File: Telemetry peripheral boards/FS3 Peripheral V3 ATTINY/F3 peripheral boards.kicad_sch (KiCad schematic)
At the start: 49 parts, among them J1 ATS668LSM, J2 Exit Connector, J3 Potentiometer, J4 Strain Gauge, J5 Tire temp Sensor, J6 1x1 Tire Air Temp Sensor, J7 1x8 Tire Surface Temp Sensor, U1 LM2907M/NOPB, U2 INA125U, U3 MCP2515-I/SO, U4 ISO1050DUB, U5 ATtiny1616-S, U6 LM7805CV, U7 LF33CV, Y1 STDCSU1-8M

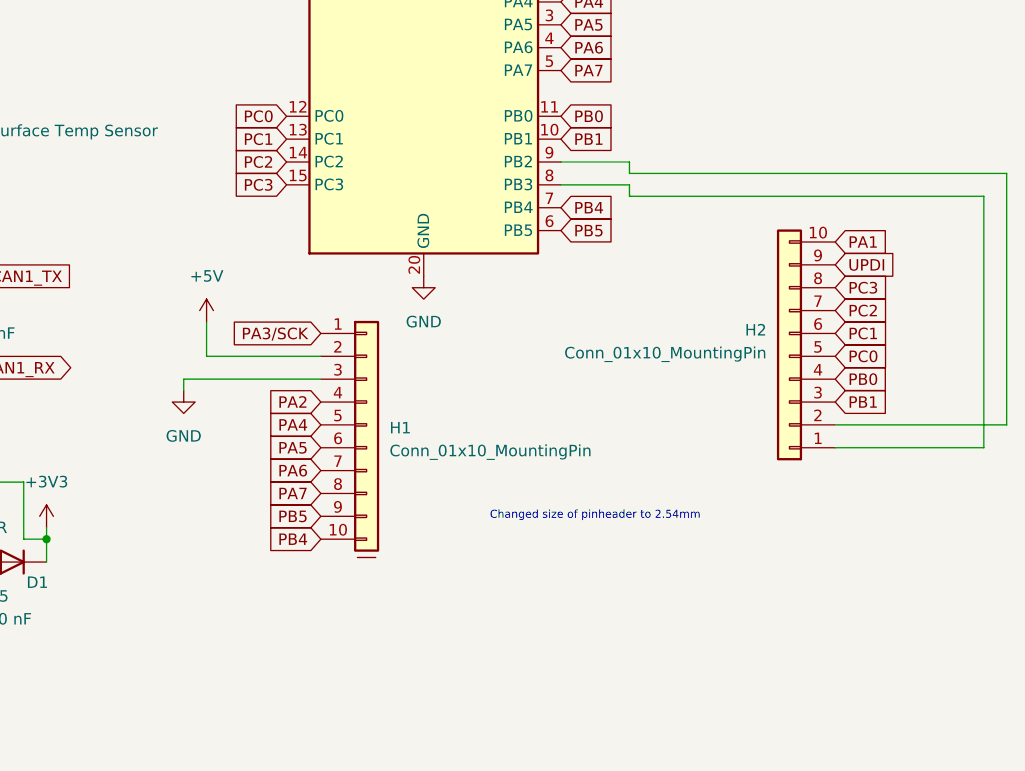
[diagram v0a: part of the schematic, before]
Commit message: updated schematic
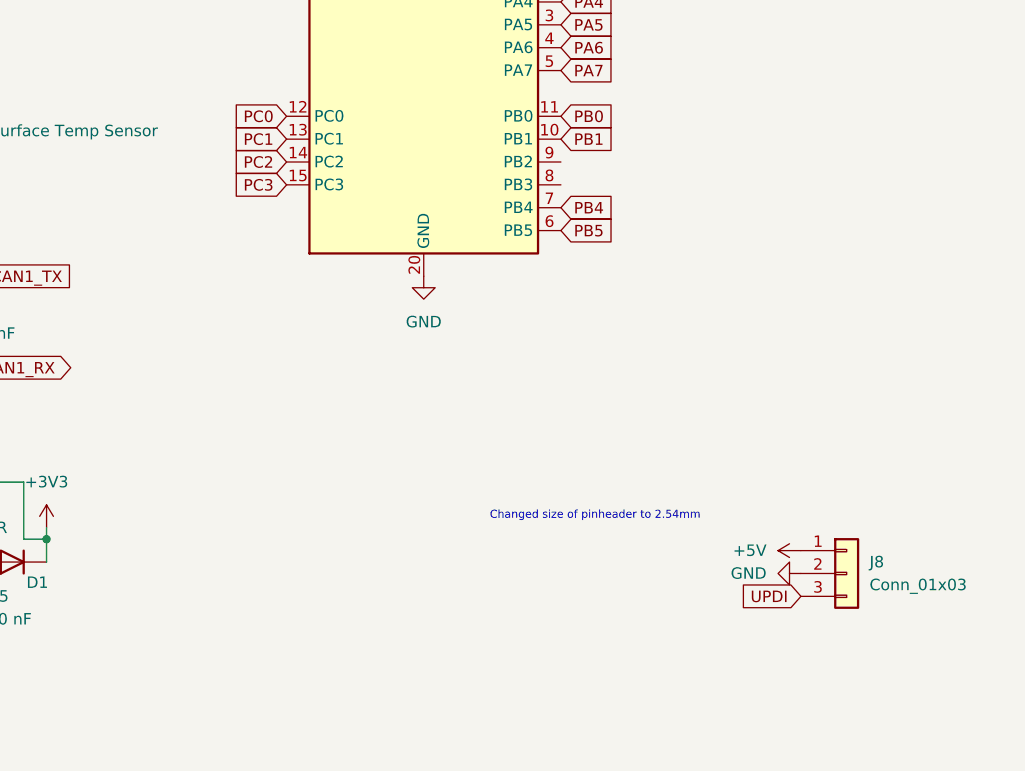
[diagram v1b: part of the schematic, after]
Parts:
- removed H1, H2: Conn_01x10_MountingPin, Connector_PinHeader_2.54mm:PinHeader_1x10_P2.54mm_Vertical, symbol Connector_Generic_MountingPin:Conn_01x10_MountingPin
- added J8: Conn_01x03, Connector_PinHeader_2.54mm:PinHeader_1x03_P2.54mm_Vertical, symbol Connector_Generic:Conn_01x03
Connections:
- net +5V: now also J8.1 (Pin_1)
- net GND: now also J8.2 (Pin_2)
- net UPDI: now also J8.3 (Pin_3)

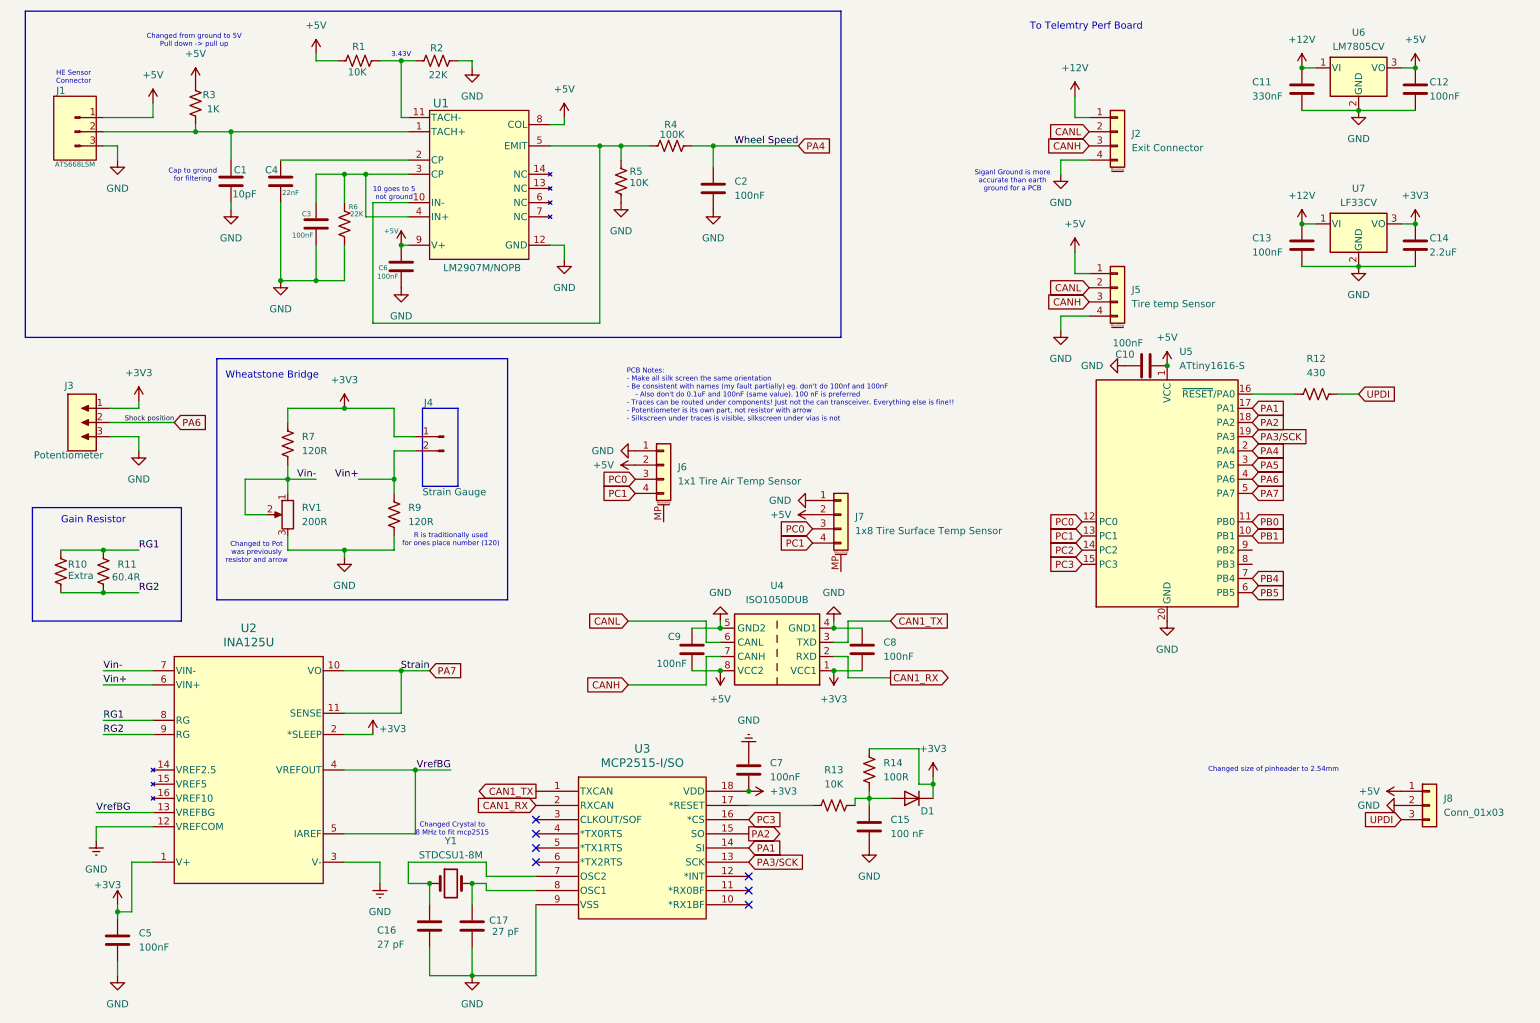
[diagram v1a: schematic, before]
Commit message: added testing pin headers and made pin change on attiny v3
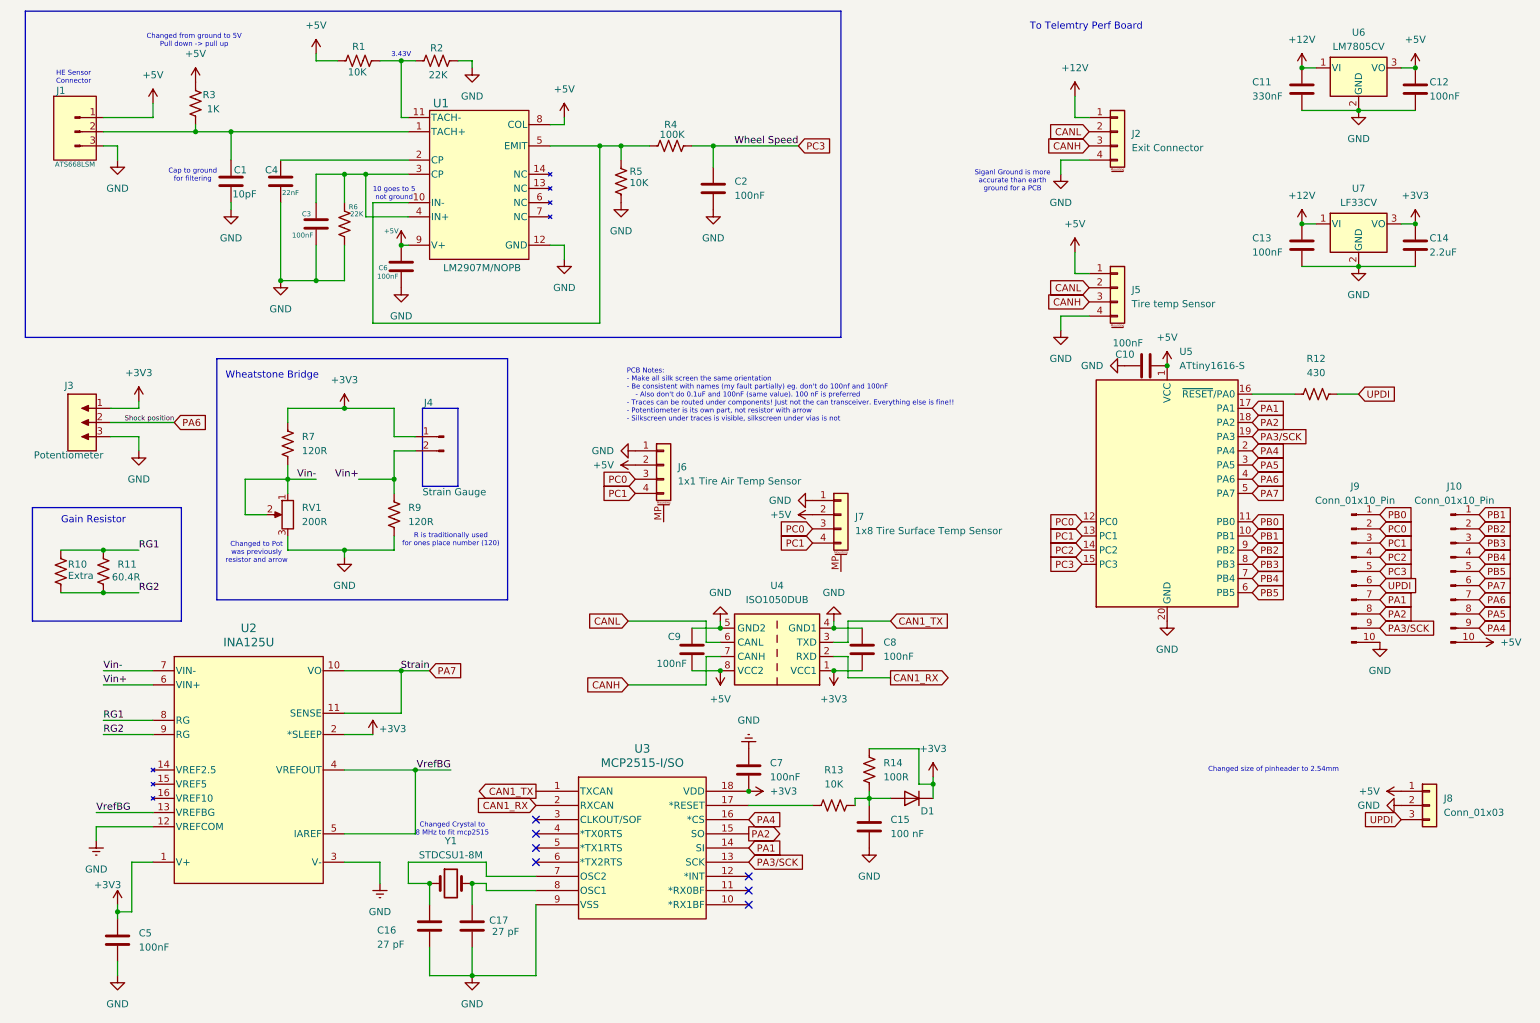
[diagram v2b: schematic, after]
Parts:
- added J10, J9: Conn_01x10_Pin, Connector_PinHeader_2.00mm:PinHeader_1x10_P2.00mm_Vertical, symbol Connector:Conn_01x10_Pin
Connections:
- net +5V: now also J10.10 (Pin_10)
- net GND: now also J9.10 (Pin_10)
- net PA1: now also J9.7 (Pin_7)
- net PA2: now also J9.8 (Pin_8)
- net PA3/SCK: now also J9.9 (Pin_9)
- net PA4: now also U3.16 (*CS), J10.9 (Pin_9); no longer C2.1, R4.2
- net PA5: now also J10.8 (Pin_8)
- net PA6: now also J10.7 (Pin_7)
- net PA7: now also J10.6 (Pin_6)
- net PB0: now also J9.1 (Pin_1)
- net PB1: now also J10.1 (Pin_1)
- net PB4: now also J10.4 (Pin_4)
- net PB5: now also J10.5 (Pin_5)
- net PC0: now also J9.2 (Pin_2)
- net PC1: now also J9.3 (Pin_3)
- net PC2: now also J9.4 (Pin_4)
- net PC3: now also C2.1, R4.2, J9.5 (Pin_5); no longer U3.16 (*CS)
- net UPDI: now also J9.6 (Pin_6)
- net PB3: now reaches U5.8 (PB3)
- net PB3: now also J10.3 (Pin_3)
- net PB2: now reaches U5.9 (PB2)
- net PB2: now also J10.2 (Pin_2)

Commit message: fixed attiny v3
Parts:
- J10, J9: footprint Connector_PinHeader_2.00mm:PinHeader_1x10_P2.00mm_Vertical -> Connector_PinHeader_2.54mm:PinHeader_1x10_P2.54mm_Vertical
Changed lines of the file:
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@@
 			)
 		)
-		(property "Footprint" "Connector_PinHeader_2.00mm:PinHeader_1x10_P2.00mm_Vertical"
+		(property "Footprint" "Connector_PinHeader_2.54mm:PinHeader_1x10_P2.54mm_Vertical"
 			(at 269.24 114.3 0)
 			(effects
@@
 			)
 		)
-		(property "Footprint" "Connector_PinHeader_2.00mm:PinHeader_1x10_P2.00mm_Vertical"
+		(property "Footprint" "Connector_PinHeader_2.54mm:PinHeader_1x10_P2.54mm_Vertical"
 			(at 251.46 114.3 0)
 			(effects
